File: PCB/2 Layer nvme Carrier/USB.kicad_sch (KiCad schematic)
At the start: 18 parts, among them J2 USB_A_Stacked, J3 USB3_A, J78 USB_A, U3 ULC0524P, U4 ULC0524P

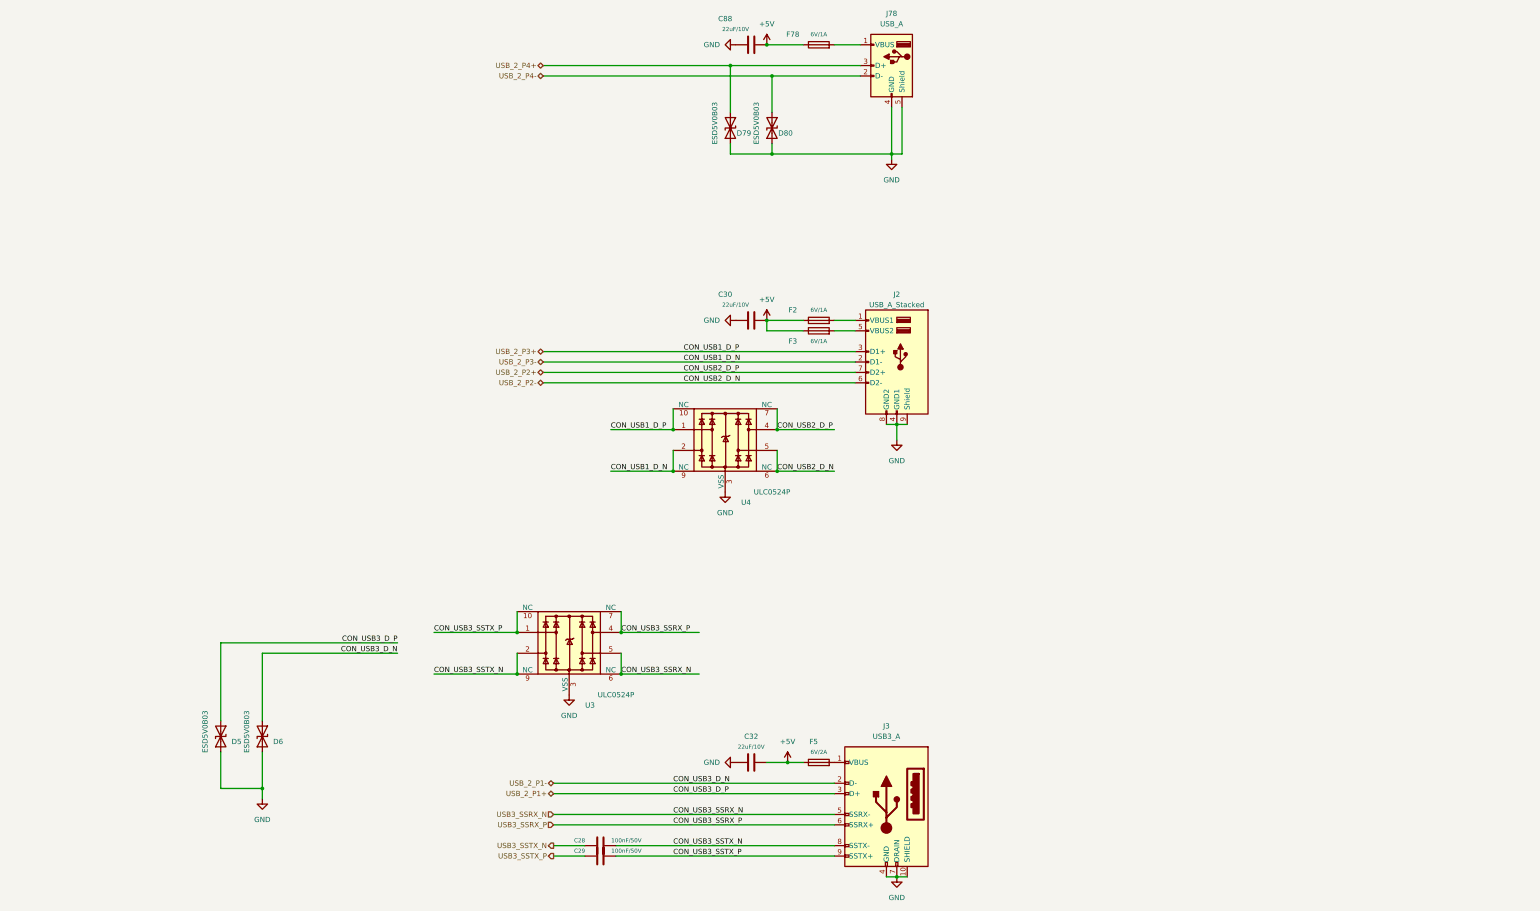
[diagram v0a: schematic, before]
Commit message: Work
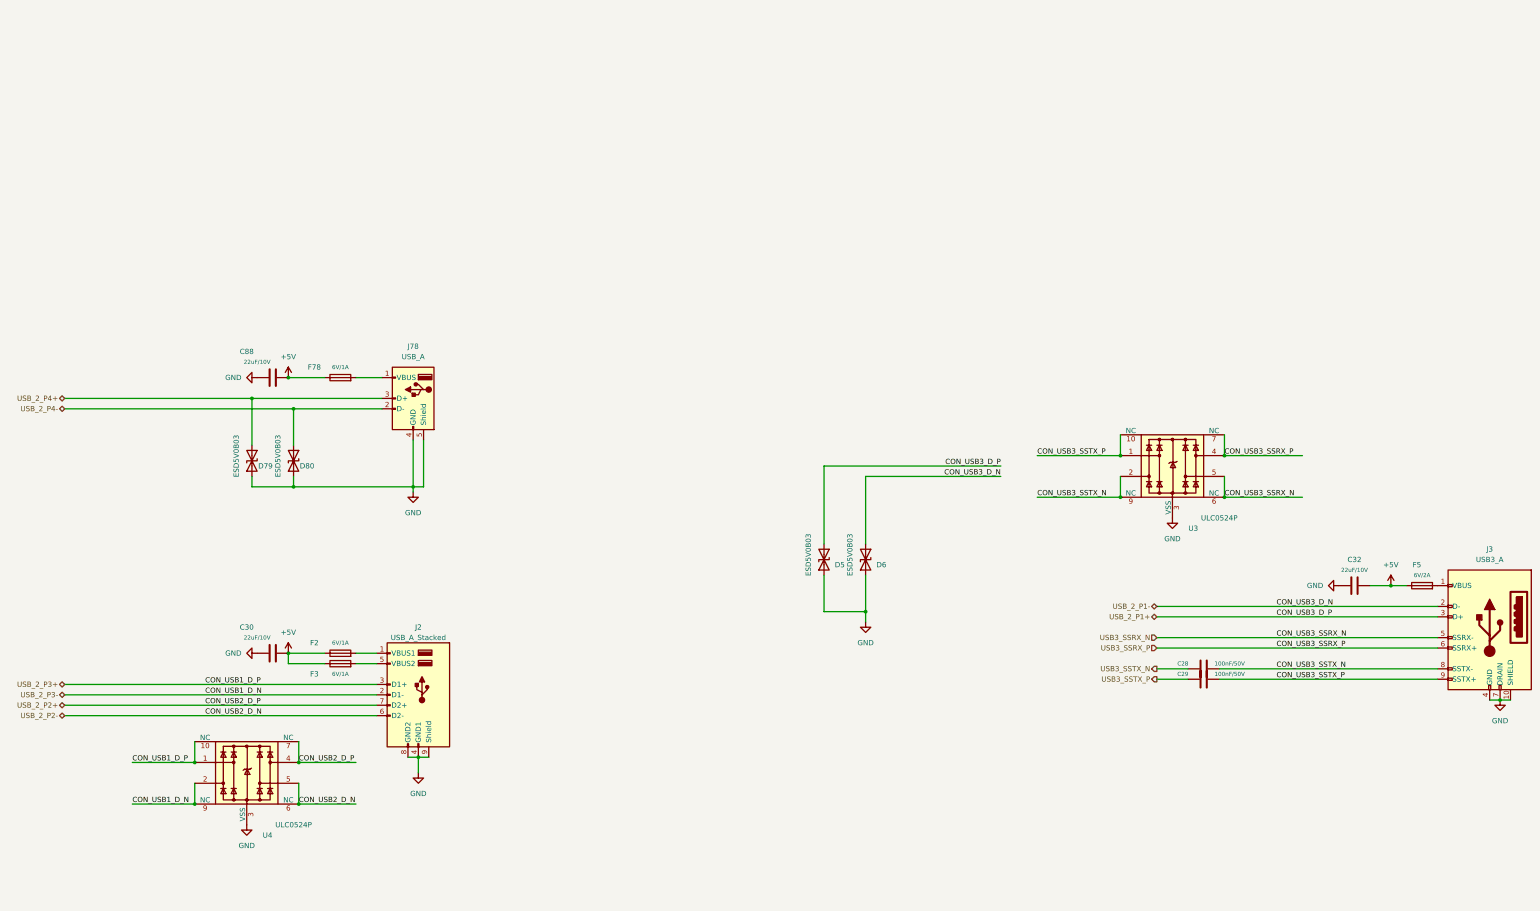
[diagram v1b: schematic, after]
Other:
- moved on the sheet: C28, C29, C30, C32, C88, D5, D6, D79, D80, F2, F3, F5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
